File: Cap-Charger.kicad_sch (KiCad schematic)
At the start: 23 parts, among them J8 Conn_01x04, J9 Conn_01x03, Q9 IRF7493

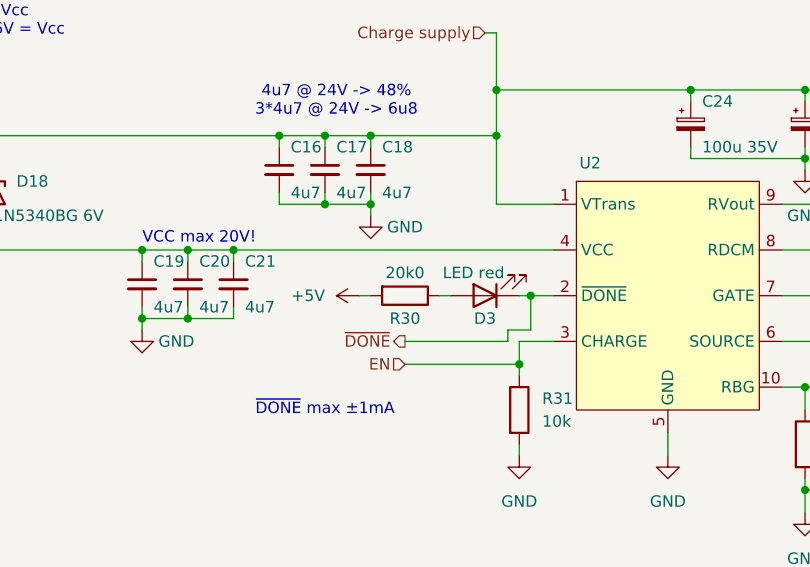
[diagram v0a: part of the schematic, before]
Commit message: rough placement
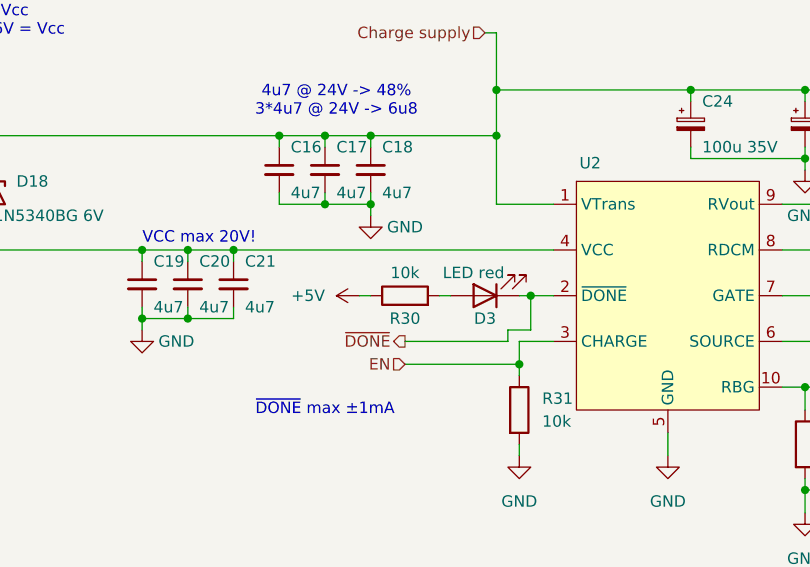
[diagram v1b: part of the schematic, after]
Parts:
- R27: footprint Resistor_SMD:R_0805_2012Metric_Pad1.20x1.40mm_HandSolder -> Resistor_SMD:R_0603_1608Metric_Pad0.98x0.95mm_HandSolder; MPN RC0805FR-0743KL -> RC0603FR-0743KL
- R29: footprint Resistor_SMD:R_0805_2012Metric_Pad1.20x1.40mm_HandSolder -> Resistor_SMD:R_0603_1608Metric_Pad0.98x0.95mm_HandSolder; MPN RC0805FR-0760K4L -> RC0603FR-0760K4L
- R30: value 20k0 -> 10k; MPN RC0805FR-0720KL -> RC0805FR-0710KL
- R31: MPN (none) -> RC0805FR-0710KL
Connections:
- net +5V: now also R30.1; no longer R30.2
- net at D3.2 (A): now also R30.2; no longer R30.1
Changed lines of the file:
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@@
+	)
+	(symbol
+		(lib_id "Device:R")
+		(at 86.36 87.63 90)
+		(unit 1)
+		(exclude_from_sim no)
+		(in_bom yes)
+		(on_board yes)
+		(dnp no)
+		(property "Reference" "R30"
+			(at 86.36 90.17 90)
+			(effects
+				(font
+					(size 1.27 1.27)
+				)
+			)
+		)
+		(property "Value" "10k"
+			(at 86.36 85.09 90)
+			(effects
+				(font
+					(size 1.27 1.27)
+				)
+			)
+		)
+		(property "Footprint" "Resistor_SMD:R_0805_2012Metric_Pad1.20x1.40mm_HandSolder"
+			(at 86.36 89.408 90)
+			(effects
+				(font
+					(size 1.27 1.27)
+				)
+				(hide yes)
+			)
+		)
+		(property "Datasheet" "~"
+			(at 86.36 87.63 0)
+			(effects
+				(font
+					(size 1.27 1.27)
+				)
+				(hide yes)
+			)
+		)
+		(property "Description" "Resistor"
+			(at 86.36 87.63 0)
+			(effects
+				(font
+					(size 1.27 1.27)
+				)
+				(hide yes)
+			)
+		)
+		(property "MPN" "RC0805FR-0710KL"
+			(at 86.36 87.63 90)
+			(effects
+				(font
+					(size 1.27 1.27)
+				)
+				(hide yes)
+			)
+		)
+		(pin "2"
+		)
+		(pin "1"
+		)
+		(instances
+			(project "Gaus-Beschleuniger"
+				(path "/10afecde-cced-4b16-9a8f-ba25affe517e/89601b47-33d3-45bd-90a7-6d36528e5bd8"
+					(reference "R30")
+					(unit 1)
+				)
+			)
+		)
 	)
 	(symbol
@@
 		(pin "1"
 		)
+		(pin "3"
+		)
+		(pin "8"
+		)
+		(pin "9"
+		)
 		(instances
 			(project ""
@@
 			)
 		)
+		(property "MPN" "RC0805FR-0710KL"
+			(at 99.06 100.33 0)
+			(effects
+				(font
+					(size 1.27 1.27)
+				)
+				(hide yes)
+			)
+		)
 		(pin "2"
 		)
@@
 			)
 		)
-		(property "Footprint" "Resistor_SMD:R_0805_2012Metric_Pad1.20x1.40mm_HandSolder"
+		(property "Footprint" "Resistor_SMD:R_0603_1608Metric_Pad0.98x0.95mm_HandSolder"
 			(at 143.51 79.248 90)
 			(effects
@@
 			)
 		)
-		(property "MPN" "RC0805FR-0760K4L"
+		(property "MPN" "RC0603FR-0760K4L"
 			(at 143.51 77.47 0)
 			(effects
@@
 				(path "/10afecde-cced-4b16-9a8f-ba25affe517e/89601b47-33d3-45bd-90a7-6d36528e5bd8"
 					(reference "R29")
-					(unit 1)
-				)
-			)
-		)
-	)
-	(symbol
-		(lib_id "Device:R")
-		(at 86.36 87.63 270)
-		(unit 1)
-		(exclude_from_sim no)
-		(in_bom yes)
-		(on_board yes)
-		(dnp no)
-		(property "Reference" "R30"
-			(at 86.36 90.17 90)
-			(effects
-				(font
-					(size 1.27 1.27)
-				)
-			)
-		)
-		(property "Value" "20k0"
-			(at 86.36 85.09 90)
-			(effects
-				(font
-					(size 1.27 1.27)
-				)
-			)
-		)
-		(property "Footprint" "Resistor_SMD:R_0805_2012Metric_Pad1.20x1.40mm_HandSolder"
-			(at 86.36 85.852 90)
-			(effects
-				(font
-					(size 1.27 1.27)
-				)
-				(hide yes)
-			)
-		)
-		(property "Datasheet" "~"
-			(at 86.36 87.63 0)
-			(effects
-				(font
-					(size 1.27 1.27)
-				)
-				(hide yes)
-			)
-		)
-		(property "Description" "Resistor"
-			(at 86.36 87.63 0)
-			(effects
-				(font
-					(size 1.27 1.27)
-				)
-				(hide yes)
-			)
-		)
-		(property "MPN" "RC0805FR-0720KL"
-			(at 86.36 87.63 0)
-			(effects
-				(font
-					(size 1.27 1.27)
-				)
-				(hide yes)
-			)
-		)
-		(pin "1"
-		)
-		(pin "2"
-		)
-		(instances
-			(project "Gaus-Beschleuniger"
-				(path "/10afecde-cced-4b16-9a8f-ba25affe517e/89601b47-33d3-45bd-90a7-6d36528e5bd8"
-					(reference "R30")
 					(unit 1)
 				)
@@
 			)
 		)
-		(property "Footprint" "Resistor_SMD:R_0805_2012Metric_Pad1.20x1.40mm_HandSolder"
+		(property "Footprint" "Resistor_SMD:R_0603_1608Metric_Pad0.98x0.95mm_HandSolder"
 			(at 135.89 84.328 90)
 			(effects
@@
 			)
 		)
-		(property "MPN" "RC0805FR-0743KL"
+		(property "MPN" "RC0603FR-0743KL"
 			(at 135.89 82.55 0)
 			(effects
